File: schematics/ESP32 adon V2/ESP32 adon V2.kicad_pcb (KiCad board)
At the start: 2 copper layers, 42.5 x 66.3 mm, 38 parts, among them J1 Conn_01x08_Pin, J2 Conn_01x08_Pin, J3 Conn_01x02_Pin, J4 Conn_01x08_Pin, J5 Conn_01x08_Pin, J6 USB4215-03-A_REVA, J7 Conn_01x04_Pin, J8 Conn_01x02_Socket, Q4 MMBT7002K, Q5 MMBT7002K, Q6 MMBT7002K, SW2 SW_Push, U1 ESP32-C6-WROOM-1, U2 TCA9535DBR, U3 ADS1115IDGS, U4 TLV75733PDBV, U6 MLX90395KDC-BBA-101-RE

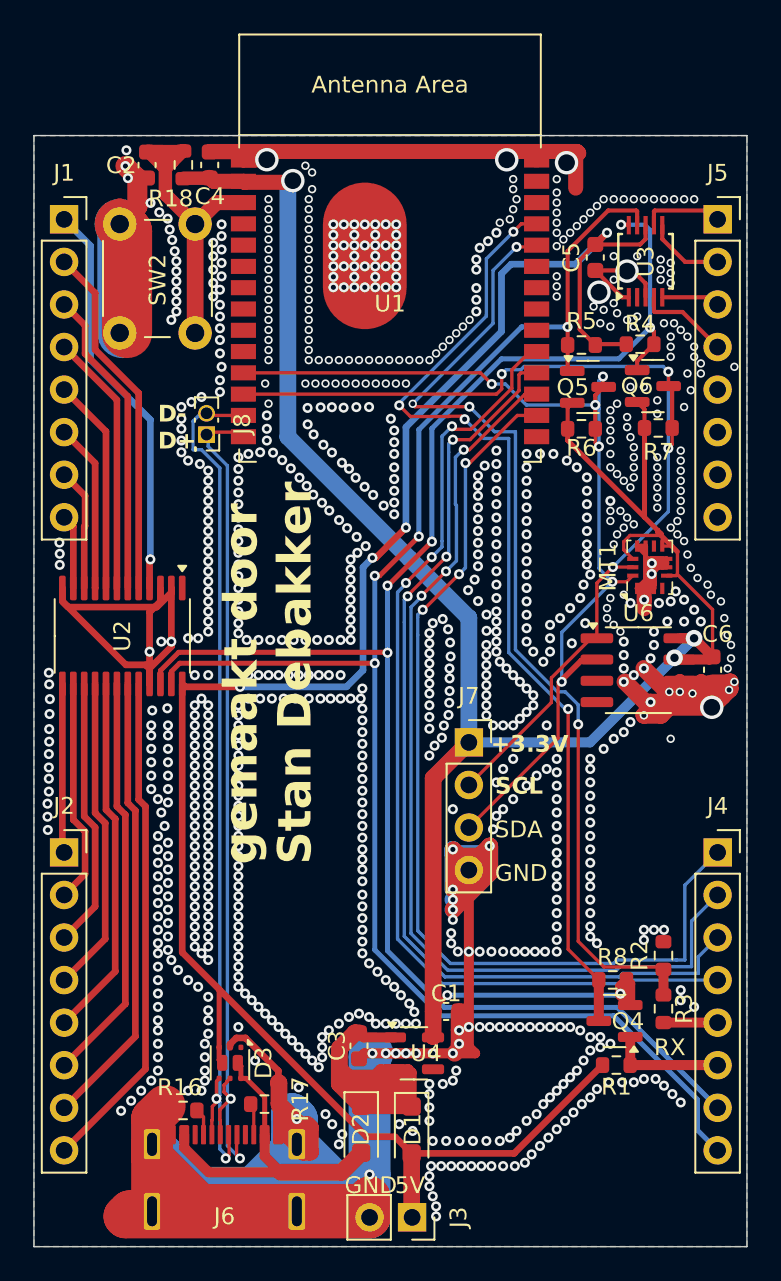
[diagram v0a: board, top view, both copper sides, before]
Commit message: verbeterde pcb layout
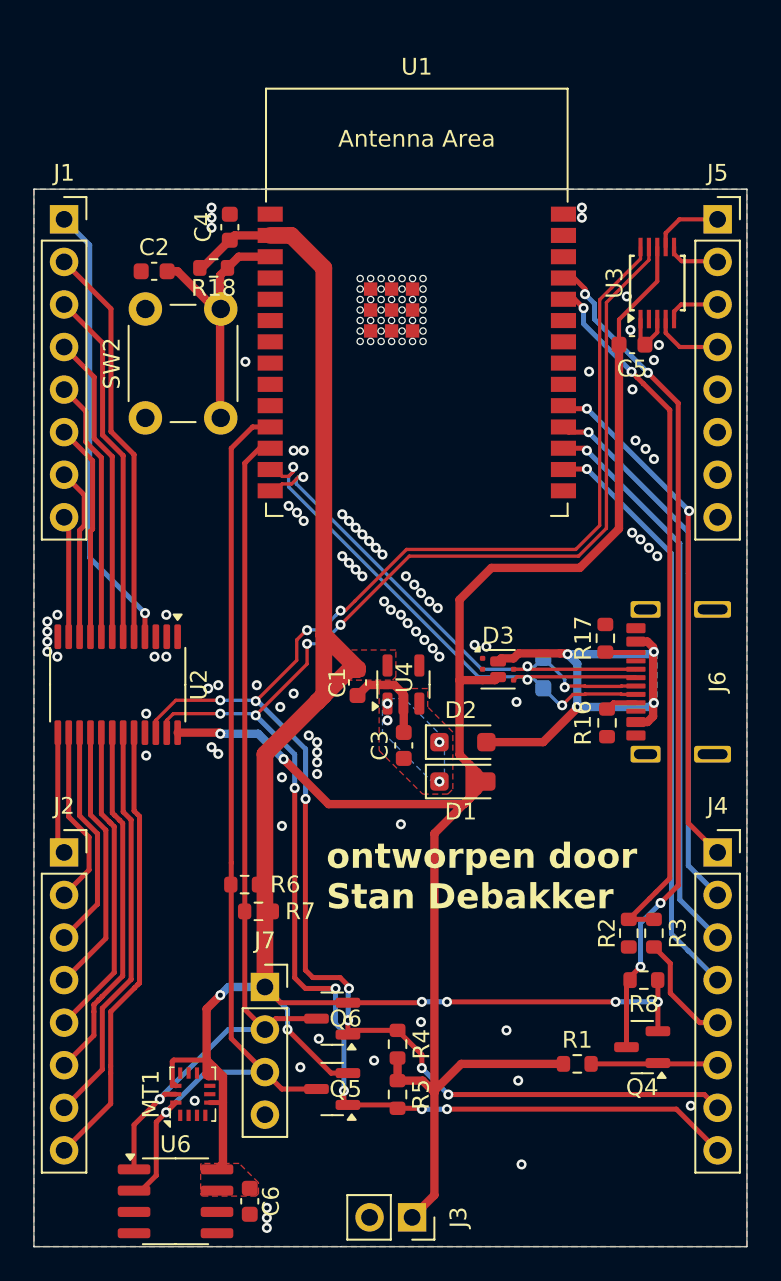
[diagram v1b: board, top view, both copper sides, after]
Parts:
- J8: value Conn_01x02_Socket -> Conn_01x02_Pin; footprint Connector_PinSocket_1.27mm:PinSocket_2x01_P1.27mm_Vertical -> Resistor_SMD:R_0603_1608Metric_Pad0.98x0.95mm_HandSolder; moved to B.Cu
- moved R5 46.1 mm to (71.7, 107.2), turned to 90 degrees
- moved J6 45.9 mm to (92.6, 82.6), turned to 90 degrees
- moved Q5 44.6 mm to (67.8, 106.9), turned to 180 degrees
- moved R4 44.2 mm to (71.7, 104.2), turned to -90 degrees
- moved Q6 42.3 mm to (67.8, 102.7), turned to 180 degrees
- moved C6 42.1 mm to (62.9, 113.6)
- moved U6 42.0 mm to (58.5, 113.6)
- moved MT1 41.6 mm to (59.5, 107.2)
- moved R7 37.4 mm to (63.4, 96.3), turned to 0 degrees
- moved R17 34.4 mm to (84.1, 80.0), turned to -90 degrees
- moved R16 34.3 mm to (84.2, 85.0), turned to 90 degrees
- moved R6 33.8 mm to (62.6, 94.7), turned to 0 degrees
- moved D3 28.4 mm to (77.7, 81.8), turned to 0 degrees
- moved J8 24.6 mm to (80.4, 82.1), turned to 90 degrees
- moved D2 23.9 mm to (75.6, 86.2), turned to 0 degrees
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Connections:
- net Net-(D1-K) renamed /Vin_reg
- D3 pad 1: unconnected-(D3-Pad1) -> GND
- J8 pad 1: /D+ -> /D-
- J8 pad 2: /D- -> /D+
- MT1 pad 10: GND -> unconnected-(MT1-RESV-Pad10)_3
- MT1 pad 11: GND -> unconnected-(MT1-RESV-Pad10)_2
- U1 pad 16: Net-(J4-Pin_1) -> Net-(J4-Pin_4)
- U1 pad 17: Net-(J4-Pin_2) -> Net-(J4-Pin_3)
- U1 pad 18: Net-(J4-Pin_3) -> Net-(J4-Pin_2)
- U1 pad 19: Net-(J4-Pin_4) -> Net-(J4-Pin_1)
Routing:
- net GND: track 271.2 -> 9.00 mm, vias 943 -> 129
- net /Vin_reg: track 31.5 -> 0.00 mm, vias 0 -> 4
- net Net-(J4-Pin_1): track 58.6 -> 31.2 mm, vias 3 -> 2
- net Net-(J4-Pin_2): track 58.6 -> 32.4 mm, vias 3 -> 1
- net Net-(J4-Pin_3): track 59.3 -> 33.7 mm, vias 3 -> 1
- net Net-(J4-Pin_4): track 59.9 -> 35.1 mm, vias 3 -> 1
- net Net-(U1-U0RXD/GPIO17): track 59.6 -> 42.5 mm, vias 4 -> 2
- net /D-: track 53.4 -> 36.8 mm, vias 2 -> 3
- net /D+: track 52.0 -> 36.3 mm, vias 2 -> 3
- net +3.3V: track 131.5 -> 117.8 mm, vias 5 -> 6
- net +5Vin: track 20.2 -> 30.8 mm, vias 0 -> 4
- net +5V: track 115.9 -> 106.7 mm, vias 4 -> 2
- net /SCL_{3.3V}: track 62.4 -> 53.5 mm, vias 4 -> 1
- net Net-(Q4-S): track 59.2 -> 50.4 mm
- net /SDA_{3.3V}: track 64.3 -> 57.9 mm, vias 6 -> 1
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- added copper zone on F.Cu, net +3.3V
- added copper zone on B.Cu, net +5Vin
- added copper zone on B.Cu, net /Vin_reg
- added copper zone on F.Cu, net /Vin_reg
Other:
- board size 42.5 x 66.3 mm -> 42.5 x 63.1 mm
- board text added: "ontworpen door Stan Debakker"
- board text removed: "+3.3V"
- board text removed: "5V"
- board text removed: "D- D+"
- board text removed: "GND"
- board text removed: "R16"
- board text removed: "R17"
- board text removed: "RX"
- board text removed: "SCL"
- board text removed: "SDA"
- board text removed: "gemaakt door Stan Debakker"
